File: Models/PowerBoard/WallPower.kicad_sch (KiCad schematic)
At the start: 1 part

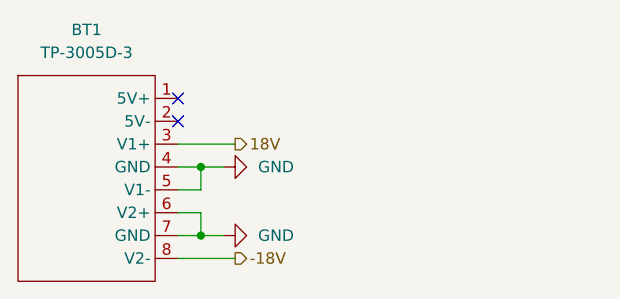
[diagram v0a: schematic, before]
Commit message: Save progress
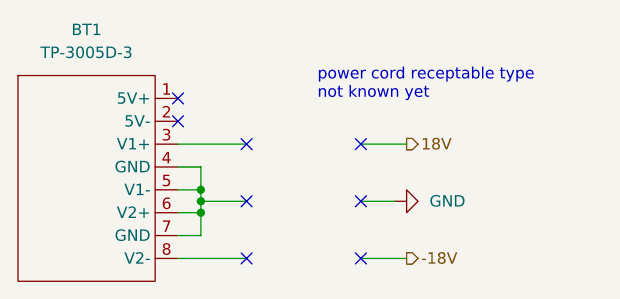
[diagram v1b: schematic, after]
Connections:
- net -18V: no longer BT1.8 (V2-)
- net 18V: no longer BT1.3 (V1+)
- net GND: no longer BT1.4 (GND), BT1.5 (V1-), BT1.6 (V2+), BT1.7 (GND)
- new net: BT1.4 (GND), BT1.5 (V1-), BT1.6 (V2+), BT1.7 (GND)
- no-connect marks 2 -> 8
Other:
- note added: "power cord receptable type not known yet"
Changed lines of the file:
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@@
 	(generator_version "9.0")
 	(paper "A4")
-	(junction
-		(at 147.32 96.52)
-		(diameter 0)
-		(color 0 0 0 0)
-	)
-	(junction
-		(at 147.32 88.9)
-		(diameter 0)
-		(color 0 0 0 0)
-	)
-	(no_connect
-		(at 144.78 81.28)
-	)
-	(no_connect
-		(at 144.78 83.82)
-	)
-	(wire
-		(pts
-			(xy 144.78 88.9) (xy 147.32 88.9)
-		)
-		(stroke
-			(width 0)
-			(type default)
-		)
-	)
-	(wire
-		(pts
-			(xy 144.78 93.98) (xy 147.32 93.98)
-		)
-		(stroke
-			(width 0)
-			(type default)
-		)
-	)
-	(wire
-		(pts
-			(xy 144.78 91.44) (xy 147.32 91.44)
-		)
-		(stroke
-			(width 0)
-			(type default)
-		)
-	)
-	(wire
-		(pts
-			(xy 147.32 88.9) (xy 149.86 88.9)
-		)
-		(stroke
-			(width 0)
-			(type default)
-		)
-	)
-	(wire
-		(pts
-			(xy 147.32 88.9) (xy 147.32 91.44)
-		)
-		(stroke
-			(width 0)
-			(type default)
-		)
-	)
-	(wire
-		(pts
-			(xy 147.32 96.52) (xy 147.32 93.98)
-		)
-		(stroke
-			(width 0)
-			(type default)
-		)
-	)
-	(wire
-		(pts
-			(xy 147.32 96.52) (xy 149.86 96.52)
-		)
-		(stroke
-			(width 0)
-			(type default)
-		)
-	)
-	(wire
-		(pts
-			(xy 144.78 99.06) (xy 151.13 99.06)
-		)
-		(stroke
-			(width 0)
-			(type default)
-		)
-	)
-	(wire
-		(pts
-			(xy 144.78 96.52) (xy 147.32 96.52)
-		)
-		(stroke
-			(width 0)
-			(type default)
-		)
-	)
-	(wire
-		(pts
-			(xy 144.78 86.36) (xy 151.13 86.36)
-		)
-		(stroke
-			(width 0)
-			(type default)
-		)
-	)
-	(hierarchical_label "-18V"
-		(shape output)
-		(at 151.13 99.06 0)
+	(text "power cord receptable type\nnot known yet"
+		(exclude_from_sim no)
+		(at 160.274 77.978 0)
 		(effects
 			(font
 				(size 1.27 1.27)
 			)
-			(justify left)
-		)
-	)
-	(hierarchical_label "18V"
+			(justify left top)
+		)
+	)
+	(junction
+		(at 147.32 91.44)
+		(diameter 0)
+		(color 0 0 0 0)
+	)
+	(junction
+		(at 147.32 93.98)
+		(diameter 0)
+		(color 0 0 0 0)
+	)
+	(junction
+		(at 147.32 92.71)
+		(diameter 0)
+		(color 0 0 0 0)
+	)
+	(no_connect
+		(at 144.78 81.28)
+	)
+	(no_connect
+		(at 165.1 86.36)
+	)
+	(no_connect
+		(at 152.4 86.36)
+	)
+	(no_connect
+		(at 165.1 99.06)
+	)
+	(no_connect
+		(at 152.4 92.71)
+	)
+	(no_connect
+		(at 165.1 92.71)
+	)
+	(no_connect
+		(at 144.78 83.82)
+	)
+	(no_connect
+		(at 152.4 99.06)
+	)
+	(wire
+		(pts
+			(xy 144.78 88.9) (xy 147.32 88.9)
+		)
+		(stroke
+			(width 0)
+			(type default)
+		)
+	)
+	(wire
+		(pts
+			(xy 147.32 92.71) (xy 152.4 92.71)
+		)
+		(stroke
+			(width 0)
+			(type default)
+		)
+	)
+	(wire
+		(pts
+			(xy 147.32 92.71) (xy 147.32 93.98)
+		)
+		(stroke
+			(width 0)
+			(type default)
+		)
+	)
+	(wire
+		(pts
+			(xy 144.78 93.98) (xy 147.32 93.98)
+		)
+		(stroke
+			(width 0)
+			(type default)
+		)
+	)
+	(wire
+		(pts
+			(xy 144.78 91.44) (xy 147.32 91.44)
+		)
+		(stroke
+			(width 0)
+			(type default)
+		)
+	)
+	(wire
+		(pts
+			(xy 165.1 86.36) (xy 170.18 86.36)
+		)
+		(stroke
+			(width 0)
+			(type default)
+		)
+	)
+	(wire
+		(pts
+			(xy 147.32 88.9) (xy 147.32 91.44)
+		)
+		(stroke
+			(width 0)
+			(type default)
+		)
+	)
+	(wire
+		(pts
+			(xy 144.78 86.36) (xy 152.4 86.36)
+		)
+		(stroke
+			(width 0)
+			(type default)
+		)
+	)
+	(wire
+		(pts
+			(xy 147.32 91.44) (xy 147.32 92.71)
+		)
+		(stroke
+			(width 0)
+			(type default)
+		)
+	)
+	(wire
+		(pts
+			(xy 165.1 92.71) (xy 168.91 92.71)
+		)
+		(stroke
+			(width 0)
+			(type default)
+		)
+	)
+	(wire
+		(pts
+			(xy 147.32 96.52) (xy 147.32 93.98)
+		)
+		(stroke
+			(width 0)
+			(type default)
+		)
+	)
+	(wire
+		(pts
+			(xy 144.78 99.06) (xy 152.4 99.06)
+		)
+		(stroke
+			(width 0)
+			(type default)
+		)
+	)
+	(wire
+		(pts
+			(xy 144.78 96.52) (xy 147.32 96.52)
+		)
+		(stroke
+			(width 0)
+			(type default)
+		)
+	)
+	(wire
+		(pts
+			(xy 165.1 99.06) (xy 170.18 99.06)
+		)
+		(stroke
+			(width 0)
+			(type default)
+		)
+	)
+	(hierarchical_label "-18V"
 		(shape output)
-		(at 151.13 86.36 0)
+		(at 170.18 99.06 0)
 		(effects
 			(font
@@
 		)
 	)
+	(hierarchical_label "18V"
+		(shape output)
+		(at 170.18 86.36 0)
+		(effects
+			(font
+				(size 1.27 1.27)
+			)
+			(justify left)
+		)
+	)
 	(symbol
 		(lib_id "power:GND")
-		(at 149.86 96.52 90)
+		(at 168.91 92.71 90)
 		(unit 1)
 		(exclude_from_sim no)
@@
 		(dnp no)
 		(fields_autoplaced yes)
-		(property "Reference" "#PWR02"
-			(at 156.21 96.52 0)
+		(property "Reference" "#PWR01"
+			(at 175.26 92.71 0)
 			(effects
 				(font
@@
 		)
 		(property "Value" "GND"
-			(at 153.67 96.5199 90)
+			(at 172.72 92.7099 90)
 			(effects
 				(font
@@
 		)
 		(property "Footprint" ""
-			(at 149.86 96.52 0)
+			(at 168.91 92.71 0)
 			(effects
 				(font
@@
 		)
 		(property "Datasheet" ""
-			(at 149.86 96.52 0)
+			(at 168.91 92.71 0)
 			(effects
 				(font
@@
 		)
 		(property "Description" "Power symbol creates a global label with name \"GND\" , ground"
-			(at 149.86 96.52 0)
+			(at 168.91 92.71 0)
 			(effects
 				(font
@@
 		)
 		(instances
-			(project "PowerBoard"
+			(project ""
 				(path "/c19e9b7b-7f36-470c-862a-1a648d3f14f6/16a77afe-3056-4f83-9f80-787a2ef93cd8"
-					(reference "#PWR02")
+					(reference "#PWR01")
 					(unit 1)
 				)
@@
 					(unit 1)
 				)
-			)
-		)
-	)
-	(symbol
-		(lib_id "power:GND")
-		(at 149.86 88.9 90)
-		(unit 1)
-		(exclude_from_sim no)
-		(in_bom yes)
-		(on_board yes)
-		(dnp no)
-		(fields_autoplaced yes)
-		(property "Reference" "#PWR01"
-			(at 156.21 88.9 0)
-			(effects
-				(font
-					(size 1.27 1.27)
-				)
-				(hide yes)
-			)
-		)
-		(property "Value" "GND"
-			(at 153.67 88.8999 90)
-			(effects
-				(font
-					(size 1.27 1.27)
-				)
-				(justify right)
-			)
-		)
-		(property "Footprint" ""
-			(at 149.86 88.9 0)
-			(effects
-				(font
-					(size 1.27 1.27)
-				)
-				(hide yes)
-			)
-		)
-		(property "Datasheet" ""
-			(at 149.86 88.9 0)
-			(effects
-				(font
-					(size 1.27 1.27)
-				)
-				(hide yes)
-			)
-		)
-		(property "Description" "Power symbol creates a global label with name \"GND\" , ground"
-			(at 149.86 88.9 0)
-			(effects
-				(font
-					(size 1.27 1.27)
-				)
-				(hide yes)
-			)
-		)
-		(pin "1"
-		)
-		(instances
-			(project ""
-				(path "/c19e9b7b-7f36-470c-862a-1a648d3f14f6/16a77afe-3056-4f83-9f80-787a2ef93cd8"
-					(reference "#PWR01")
-					(unit 1)
-				)
